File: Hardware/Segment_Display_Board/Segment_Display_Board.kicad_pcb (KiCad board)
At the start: 2 copper layers, 64.4 x 141 mm, 85 parts, among them J101 IN, J102 OUT, J301 USB_B_Micro, J302 PROG, J401 19V Input, J501 Bottom Conn, J502 Top Conn, Q1001 MMBT3904, Q1002 MMBT3906, Q1101 MMBT3904, Q1102 MMBT3906, Q1201 MMBT3904, Q1202 MMBT3906, Q601 MMBT3904, Q602 MMBT3906, Q701 MMBT3904, Q702 MMBT3906, Q801 MMBT3904, Q802 MMBT3906, Q901 MMBT3904, Q902 MMBT3906, SW201 RESET, SW202 DAY_RESET, SW203 DAY_ADV, SW204 DAY_SUB, U201 ATmega328P-A, U202 DS1307Z+, U301 FT232RL, U401 LM1117-5.0, U501 SN74HC595, Y201 16mHz, Y202 32.768kHz

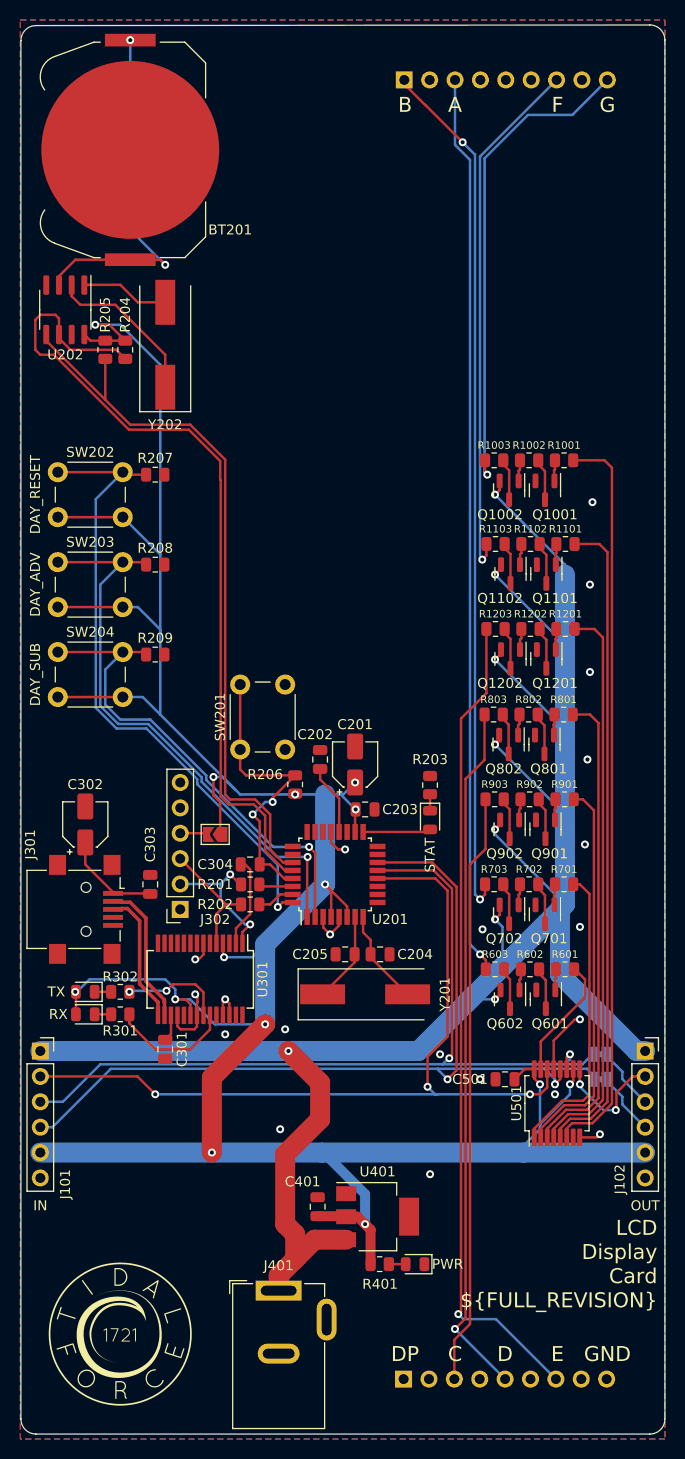
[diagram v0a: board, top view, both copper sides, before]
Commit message: Add a bunch more great stuff
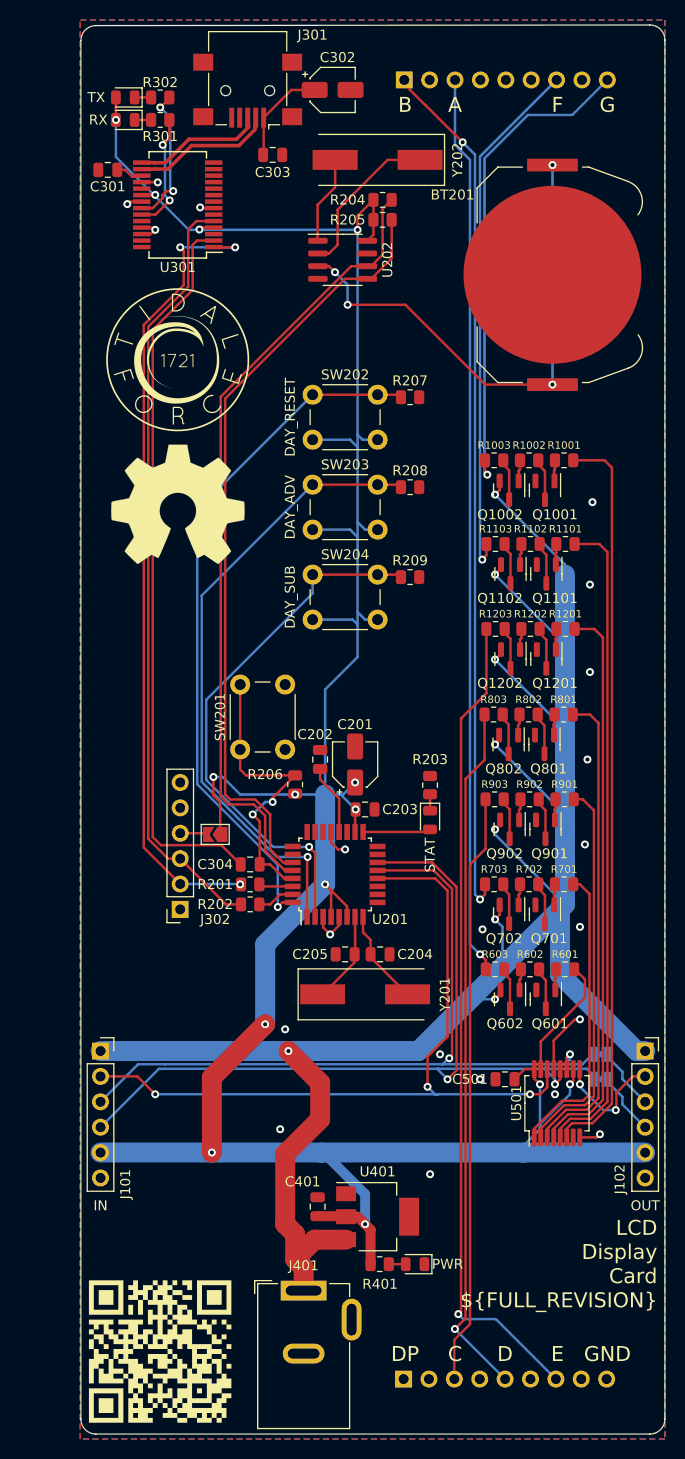
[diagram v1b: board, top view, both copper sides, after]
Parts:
- added G***: LOGO, 1721_templates:QRCODE_AccidentCounter, F.Cu at (122.5, 158.2)
- added REF**: OSHW-Symbol_13.4x12mm_SilkScreen, Symbol:OSHW-Symbol_13.4x12mm_SilkScreen, F.Cu at (124.2, 73.5)
- moved G*** 97.7 mm to (124.2, 59.0)
- moved D301 89.6 mm to (119.0, 35.0)
- moved D302 89.6 mm to (119.0, 32.8)
- moved R301 89.6 mm to (122.5, 35.0)
- moved R302 89.6 mm to (122.5, 32.8)
- moved C301 88.2 mm to (117.2, 40.0), turned to 180 degrees
- moved J301 83.5 mm to (131.2, 32.1), turned to 180 degrees
- moved C302 77.6 mm to (139.8, 32.0), turned to 0 degrees
- moved U301 77.5 mm to (124.2, 43.5), turned to 180 degrees
- moved C303 74.0 mm to (133.8, 38.5), turned to 0 degrees
- moved BT201 44.1 mm to (161.8, 50.5), turned to 90 degrees
- moved R205 30.6 mm to (144.8, 45.0), turned to 0 degrees
- moved R204 29.8 mm to (144.8, 43.0), turned to 0 degrees
- moved U202 28.2 mm to (140.8, 49.0), turned to 0 degrees
- moved Y202 28.2 mm to (144.2, 39.0), turned to 180 degrees
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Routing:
- net /MCU/RXD: track 14.7 -> 80.8 mm, vias 2 -> 3
- net /MCU/TXD: track 12.3 -> 77.5 mm
- net Net-(C304-Pad2): track 9.15 -> 73.1 mm
- net Net-(BT201-Pad1): track 36.4 -> 51.5 mm, vias 2 -> 4
- net +5V: track 303.3 -> 291.0 mm
- net +19V: track 215.8 -> 209.5 mm
- net /L_OUT: track 92.1 -> 86.1 mm
- net /D_OUT: track 82.8 -> 76.8 mm
- net /C_OUT: track 86.4 -> 80.3 mm
- net /MCU/SDA: track 72.7 -> 78.2 mm
- net /MCU/DAY_SUBTRACT: track 48.7 -> 54.2 mm
- net /MCU/DAY_ADVANCE: track 57.6 -> 63.0 mm
- net /MCU/DAY_RESET: track 64.6 -> 70.0 mm
- net GND: track 27.7 -> 22.9 mm
- net Net-(R302-Pad2): track 10.4 -> 14.3 mm
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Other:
- board size 64.4 x 141 mm -> 58.4 x 141 mm
- board text added: "Designed for FRC 1721 Tidal Force By Joe and Mark Sedutto"
